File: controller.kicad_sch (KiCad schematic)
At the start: 42 parts, among them J1 I2C, J2 EEPROM DISABLE, J3 Conn_02x18_Odd_Even, J4 5V, J5 USB_B_Mini, J6 Conn_01x05, J7 Conn_01x18, J8 GPIO, SW2 RST, U1 CY7C68013A-56PVX, U2 AZ1117-3.3, U3 CAT24C128, Y1 24MHz

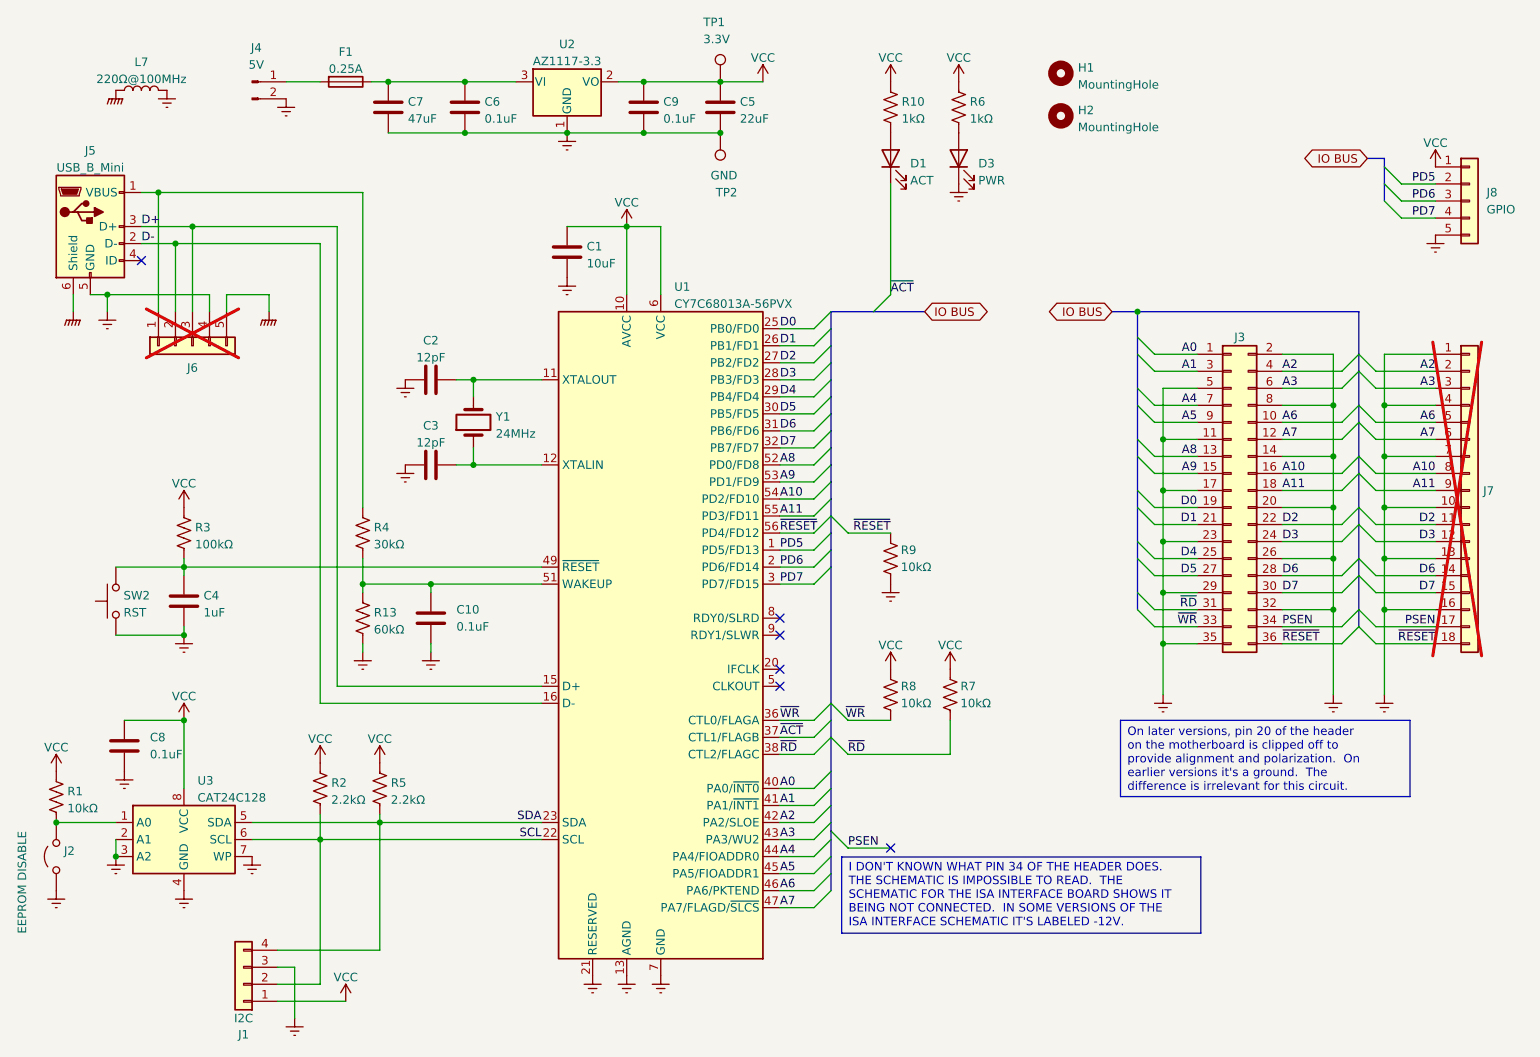
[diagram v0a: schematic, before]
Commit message: don't think I changed anything, just updated kicad
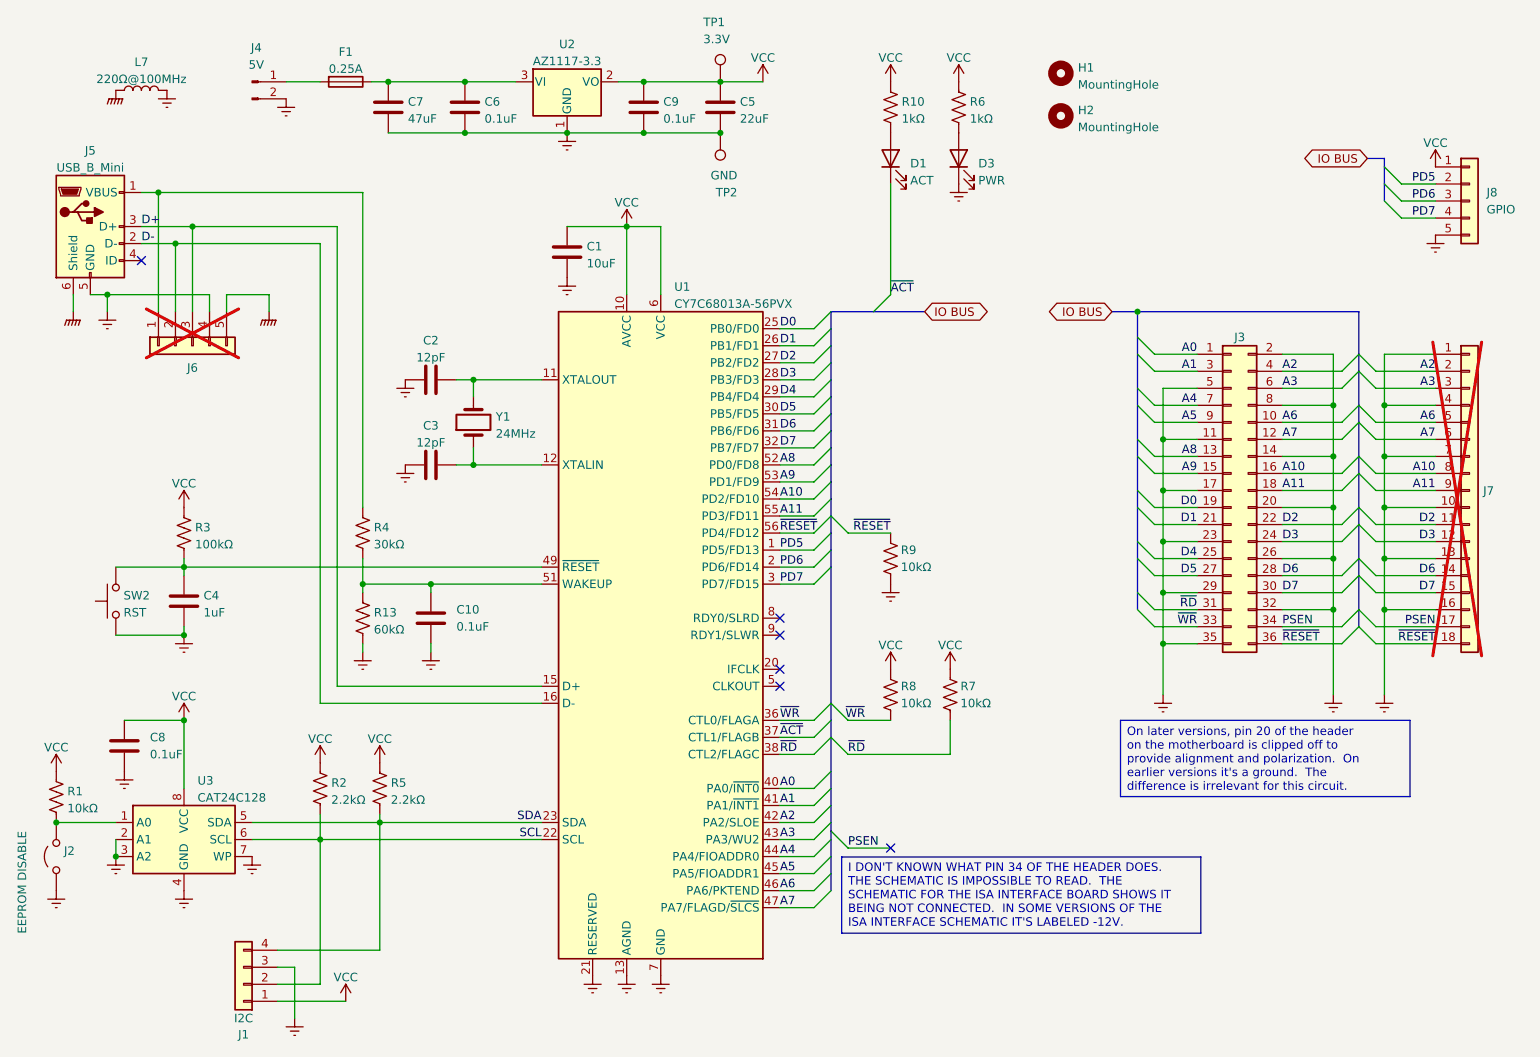
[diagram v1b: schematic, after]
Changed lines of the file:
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@@
 (kicad_sch
-	(version 20231120)
+	(version 20250114)
 	(generator "eeschema")
-	(generator_version "8.0")
+	(generator_version "9.0")
 	(paper "A4")
+	(text_box "I DON'T KNOWN WHAT PIN 34 OF THE HEADER DOES.\nTHE SCHEMATIC IS IMPOSSIBLE TO READ.  THE\nSCHEMATIC FOR THE ISA INTERFACE BOARD SHOWS IT\nBEING NOT CONNECTED.  IN SOME VERSIONS OF THE\nISA INTERFACE SCHEMATIC IT'S LABELED -12V."
+		(exclude_from_sim no)
+		(at 140.0175 147.3772 0)
+		(size 53.5797 11.3728)
+		(margins 0.9525 0.9525 0.9525 0.9525)
+		(stroke
+			(width 0)
+			(type default)
+		)
+		(fill
+			(type none)
+		)
+		(effects
+			(font
+				(size 1.27 1.27)
+			)
+			(justify left bottom)
+		)
+	)
+	(text_box "On later versions, pin 20 of the header on the motherboard is clipped off to provide alignment and polarization.  On earlier versions it's a ground.  The difference is irrelevant for this circuit."
+		(exclude_from_sim no)
+		(at 181.61 127 0)
+		(size 43.1963 11.3721)
+		(margins 0.9525 0.9525 0.9525 0.9525)
+		(stroke
+			(width 0)
+			(type default)
+		)
+		(fill
+			(type none)
+		)
+		(effects
+			(font
+				(size 1.27 1.27)
+			)
+			(justify left)
+		)
+	)
 	(junction
 		(at 110.49 39.37)
@@
 		)
 	)
-	(text_box "I DON'T KNOWN WHAT PIN 34 OF THE HEADER DOES.\nTHE SCHEMATIC IS IMPOSSIBLE TO READ.  THE\nSCHEMATIC FOR THE ISA INTERFACE BOARD SHOWS IT\nBEING NOT CONNECTED.  IN SOME VERSIONS OF THE\nISA INTERFACE SCHEMATIC IT'S LABELED -12V."
-		(exclude_from_sim no)
-		(at 140.0175 147.3772 0)
-		(size 53.5797 11.3728)
-		(stroke
-			(width 0)
-			(type default)
-		)
-		(fill
-			(type none)
-		)
-		(effects
-			(font
-				(size 1.27 1.27)
-			)
-			(justify left bottom)
-		)
-	)
-	(text_box "On later versions, pin 20 of the header on the motherboard is clipped off to provide alignment and polarization.  On earlier versions it's a ground.  The difference is irrelevant for this circuit."
-		(exclude_from_sim no)
-		(at 181.61 127 0)
-		(size 43.1963 11.3721)
-		(stroke
-			(width 0)
-			(type default)
-		)
-		(fill
-			(type none)
-		)
-		(effects
-			(font
-				(size 1.27 1.27)
-			)
-			(justify left)
-		)
-	)
 	(label "A9"
 		(at 130.81 91.44 0)
@@
 			)
 		)
+		(property "Sim.Pins" "1=K 2=A"
+			(at 147.32 43.18 0)
+			(effects
+				(font
+					(size 1.27 1.27)
+				)
+				(hide yes)
+			)
+		)
 		(pin "1"
 		)
@@
 			)
 		)
+		(property "Sim.Pins" "1=K 2=A"
+			(at 157.48 43.18 0)
+			(effects
+				(font
+					(size 1.27 1.27)
+				)
+				(hide yes)
+			)
+		)
 		(pin "1"
 		)
@@
 		)
 	)
+	(embedded_fonts no)
 )
